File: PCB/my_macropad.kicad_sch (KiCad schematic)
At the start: 8 parts, among them SW1 SW_Push, SW2 SW_Push, SW3 SW_Push, SW4 SW_Push, U1 MOUDLE-SEEEDUINO-XIAO, U2 ER_OLEDM0.91_1x-I2C

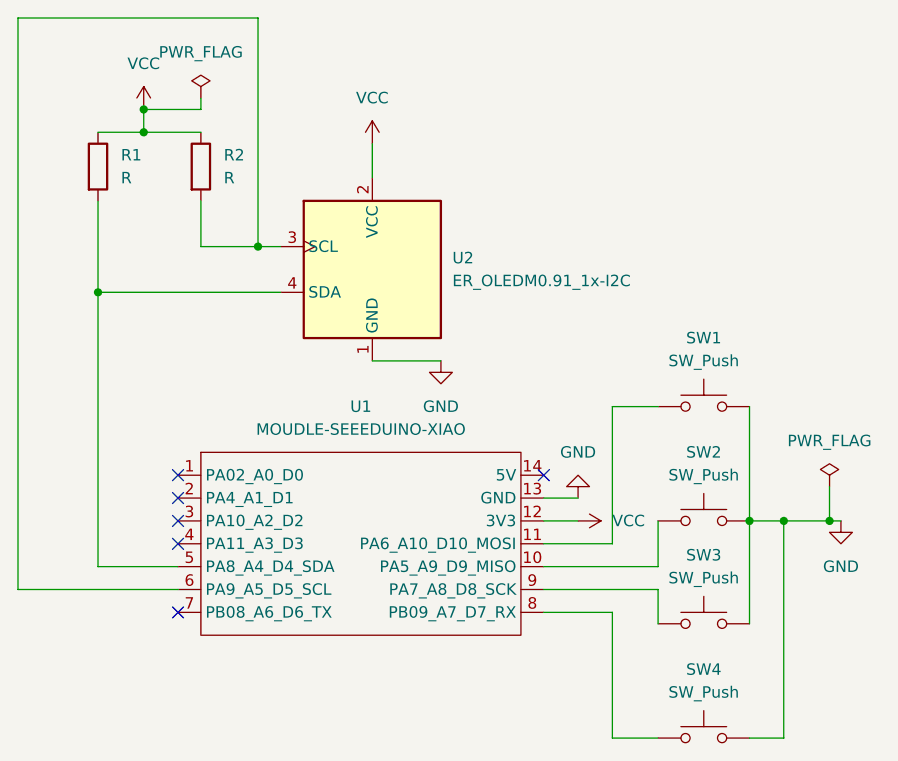
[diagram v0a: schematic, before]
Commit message: fixed changes asked
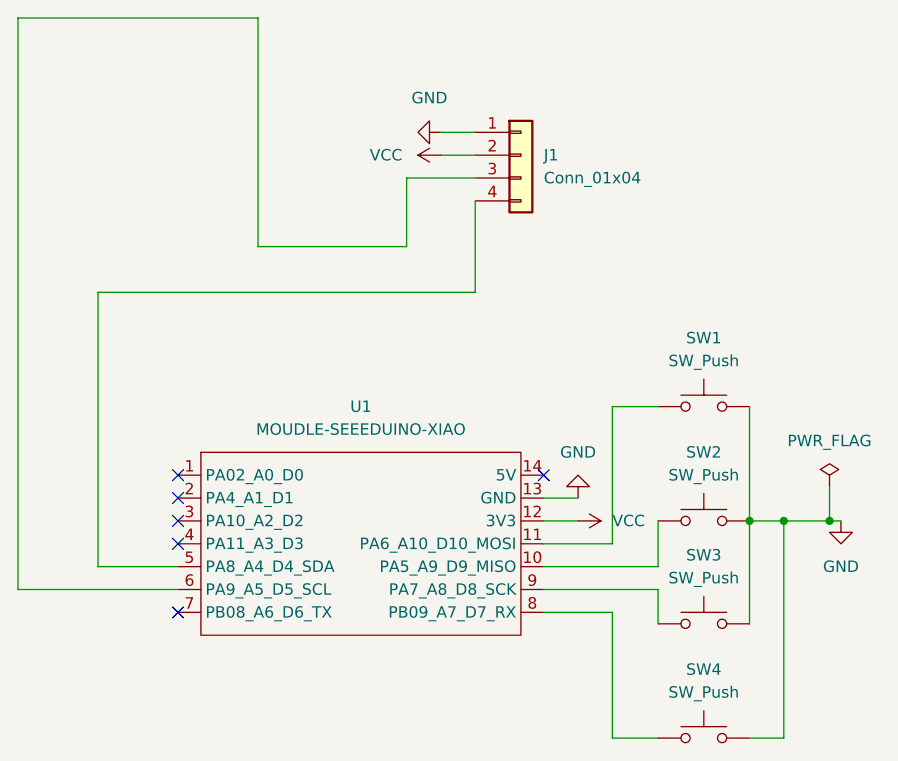
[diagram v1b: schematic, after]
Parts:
- removed R1, R2: R, Resistor_SMD:R_0805_2012Metric_Pad1.20x1.40mm_HandSolder, symbol Device:R
- removed U2: ER_OLEDM0.91_1x-I2C, KiCad-SSD1306-0.91-OLED-4pin-128x32:SSD1306-0.91-OLED-4pin-128x32, symbol Display_Graphic:ER_OLEDM0.91_1x-I2C
- added J1: Conn_01x04, KiCad-SSD1306-0.91-OLED-4pin-128x32:SSD1306-0.91-OLED-4pin-128x32, symbol Connector_Generic:Conn_01x04
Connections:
- net GND: now also J1.1 (Pin_1)
- net VCC: now also J1.2 (Pin_2)
- net at U1.6 (PA9_A5_D5_SCL): now also J1.3 (Pin_3)
- net at U1.5 (PA8_A4_D4_SDA): now also J1.4 (Pin_4)
